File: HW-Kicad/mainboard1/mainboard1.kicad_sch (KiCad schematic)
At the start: 1 part, among them M1 LightAPRS

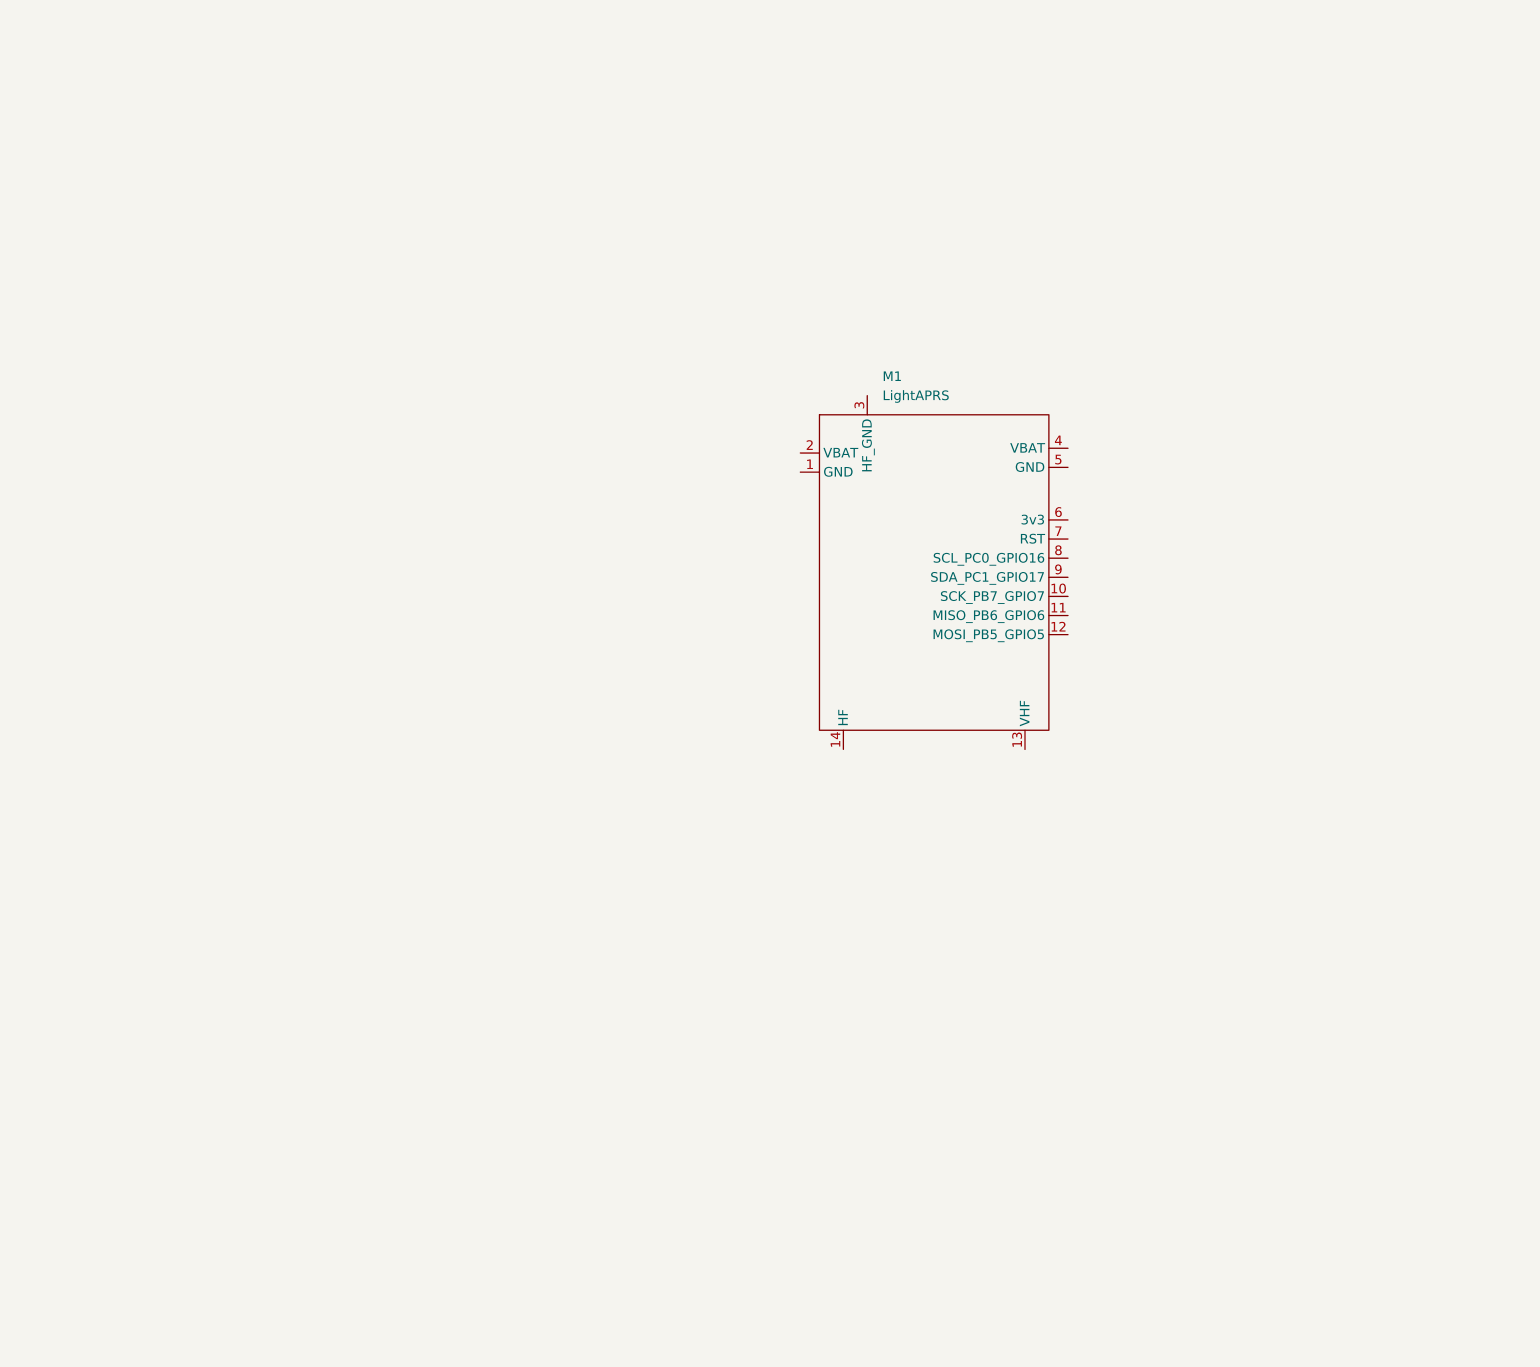
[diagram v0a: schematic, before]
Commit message: comienzo mainboard
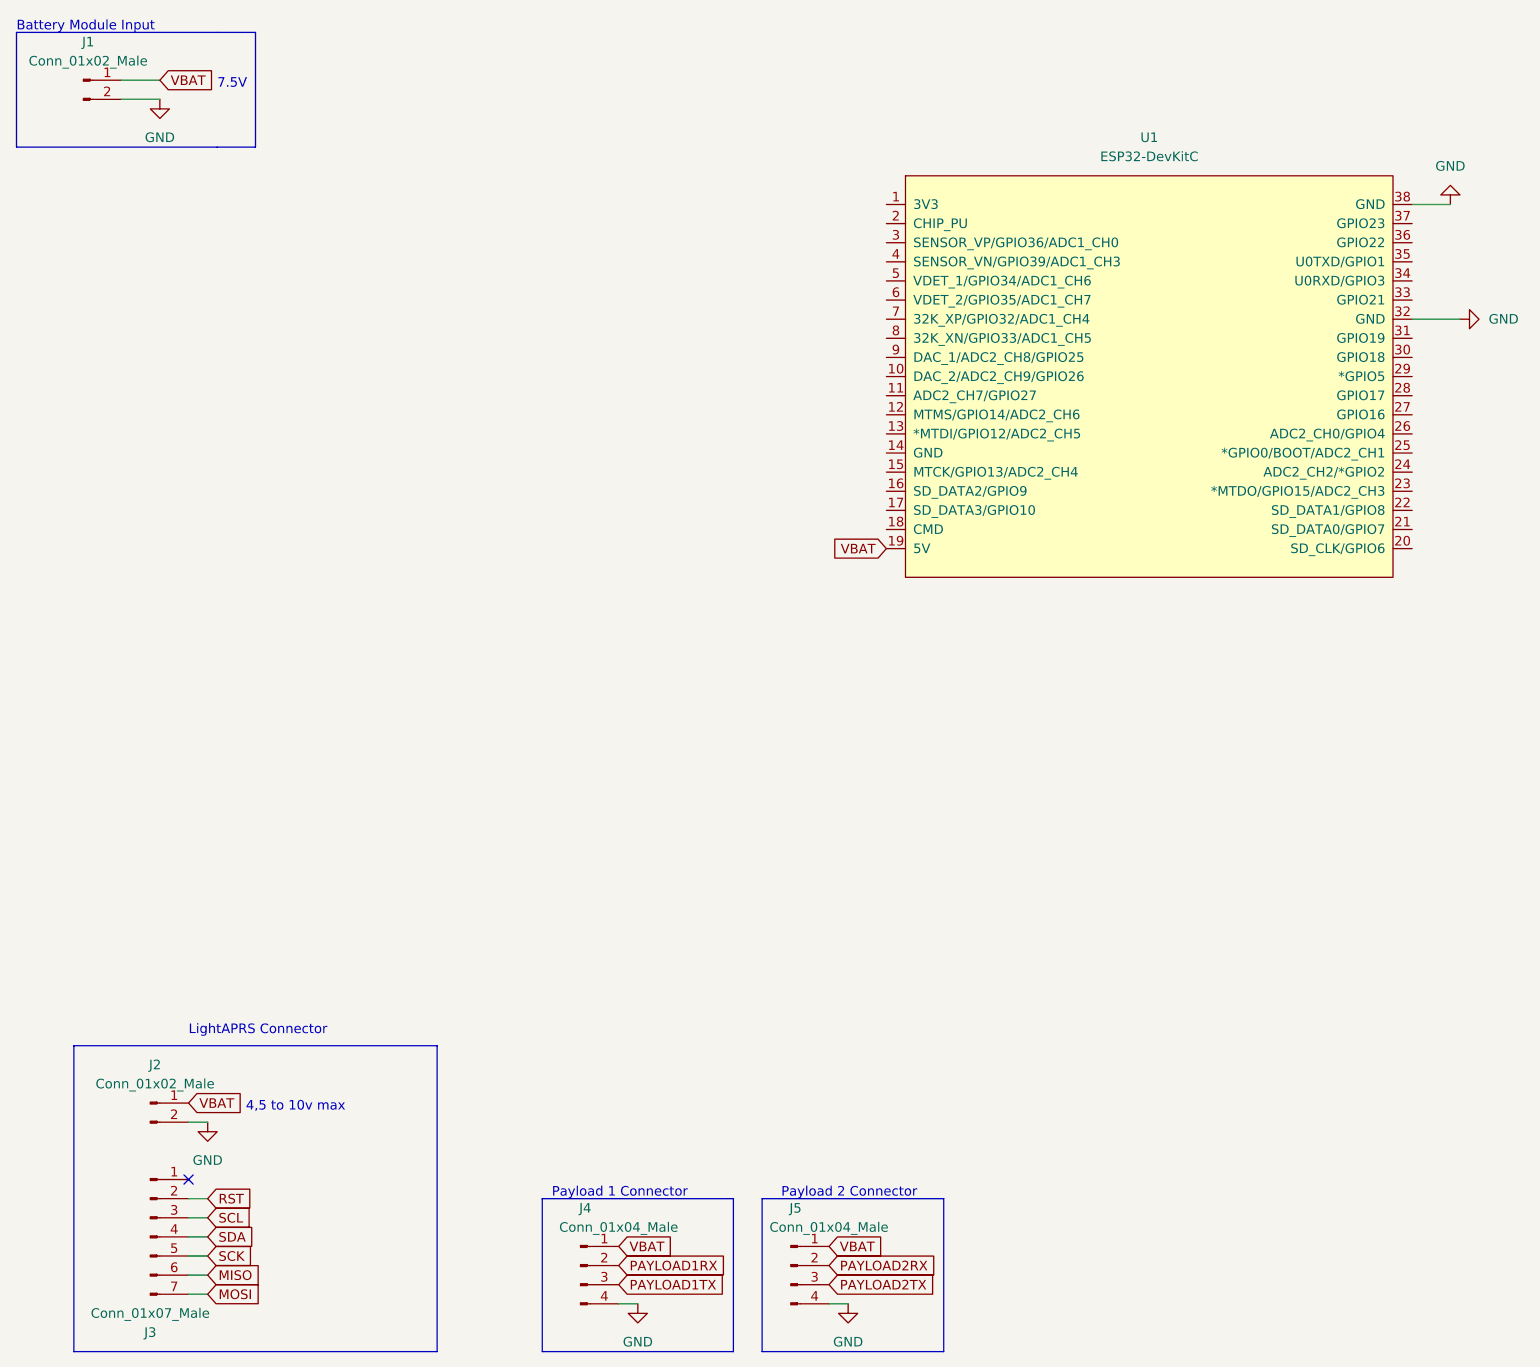
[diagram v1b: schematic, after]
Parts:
- removed M1: LightAPRS, LightAPRS:LightAPRS, symbol LightAPRS:LightAPRS
- added J1: Conn_01x02_Male, Connector_Molex:Molex_KK-254_AE-6410-02A_1x02_P2.54mm_Vertical, symbol Connector:Conn_01x02_Male
- added J2: Conn_01x02_Male, Connector_PinHeader_2.54mm:PinHeader_1x02_P2.54mm_Horizontal, symbol Connector:Conn_01x02_Male
- added J3: Conn_01x07_Male, Connector_PinHeader_2.54mm:PinHeader_1x07_P2.54mm_Horizontal, symbol Connector:Conn_01x07_Male
- added J4, J5: Conn_01x04_Male, Connector_Molex:Molex_KK-254_AE-6410-04A_1x04_P2.54mm_Vertical, symbol Connector:Conn_01x04_Male
- added U1: ESP32-DevKitC, espressif:ESP32-DevKitC, symbol Espressif:ESP32-DevKitC
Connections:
- new net GND: J1.2 (Pin_2), J2.2 (Pin_2), J4.4 (Pin_4), J5.4 (Pin_4), U1.32 (GND), U1.38 (GND)
- new net MISO: J3.6 (Pin_6)
- new net MOSI: J3.7 (Pin_7)
- new net PAYLOAD1RX: J4.2 (Pin_2)
- new net PAYLOAD1TX: J4.3 (Pin_3)
- new net PAYLOAD2RX: J5.2 (Pin_2)
- new net PAYLOAD2TX: J5.3 (Pin_3)
- new net RST: J3.2 (Pin_2)
- new net SCK: J3.5 (Pin_5)
- new net SCL: J3.3 (Pin_3)
- new net SDA: J3.4 (Pin_4)
- new net VBAT: J1.1 (Pin_1), J2.1 (Pin_1), J4.1 (Pin_1), J5.1 (Pin_1), U1.19 (5V)
- no-connect marks 0 -> 1
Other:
- note added: "4,5 to 10v max"
- note added: "7.5V"
- note added: "Battery Module Input"
- note added: "LightAPRS Connector"
- note added: "Payload 1 Connector"
- note added: "Payload 2 Connector"
